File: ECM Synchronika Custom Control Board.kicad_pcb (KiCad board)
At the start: 2 copper layers, 17 parts, among them J1 Screw_Terminal_01x03, U1 AP2112K-3.3

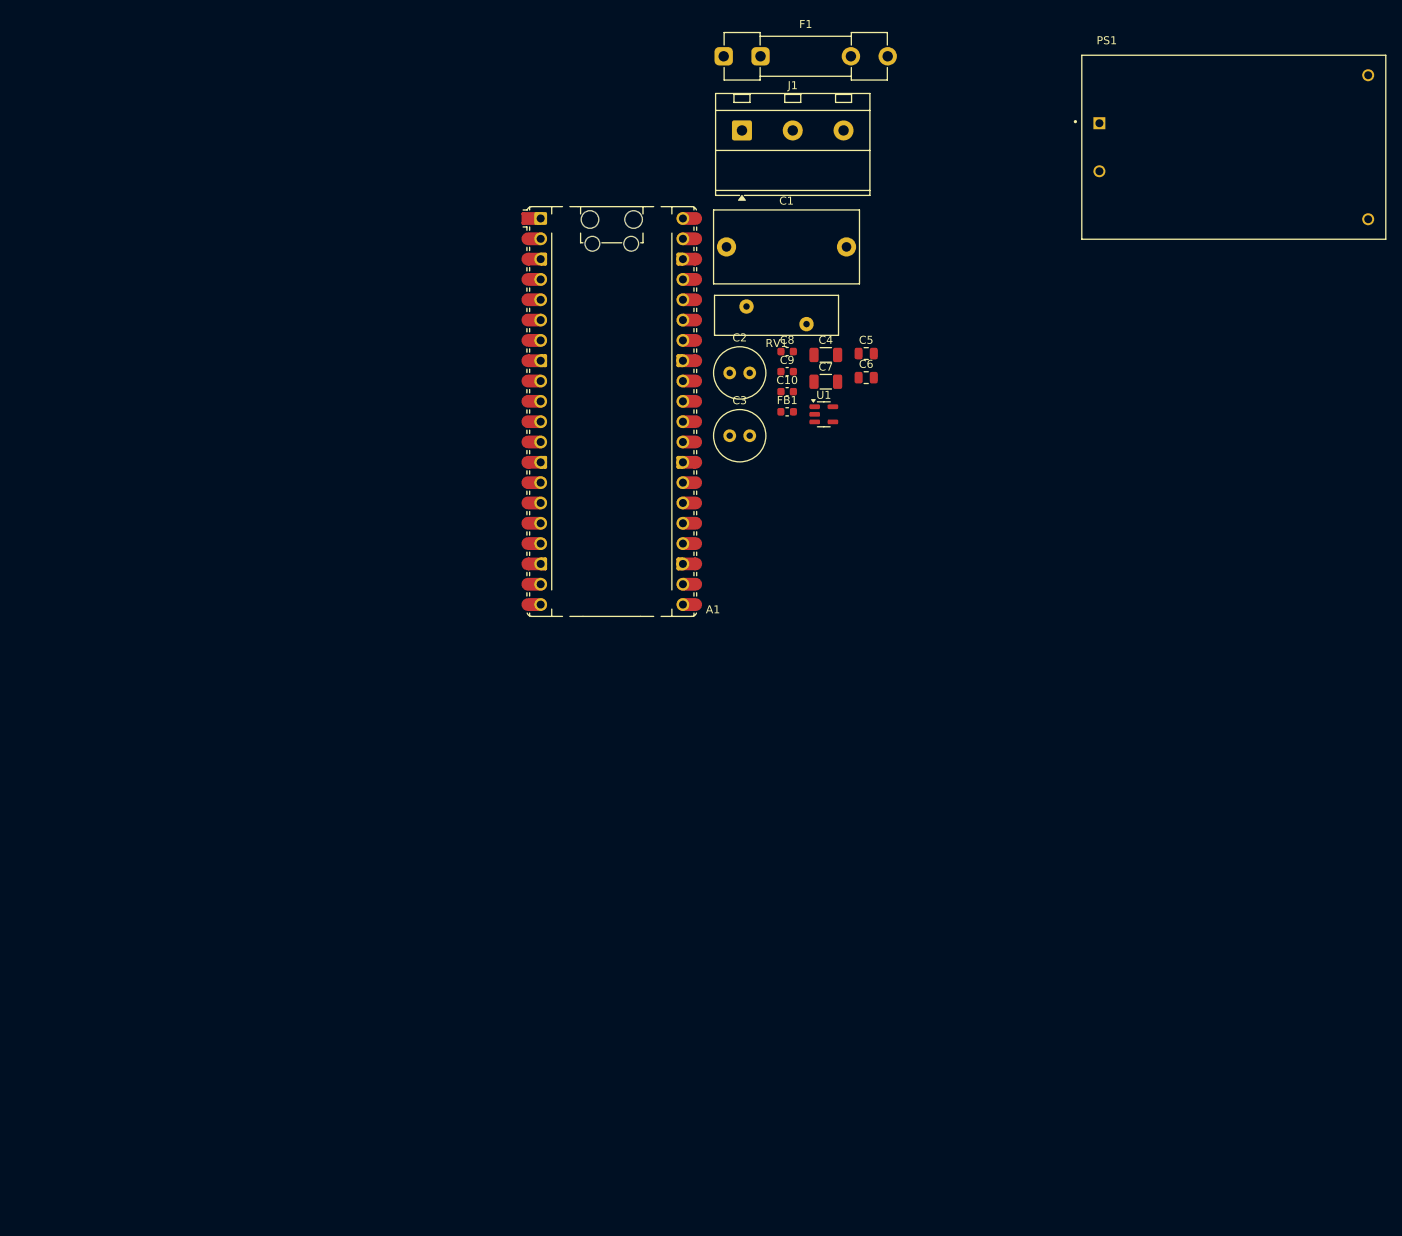
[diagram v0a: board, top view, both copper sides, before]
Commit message: Update KiCad project files
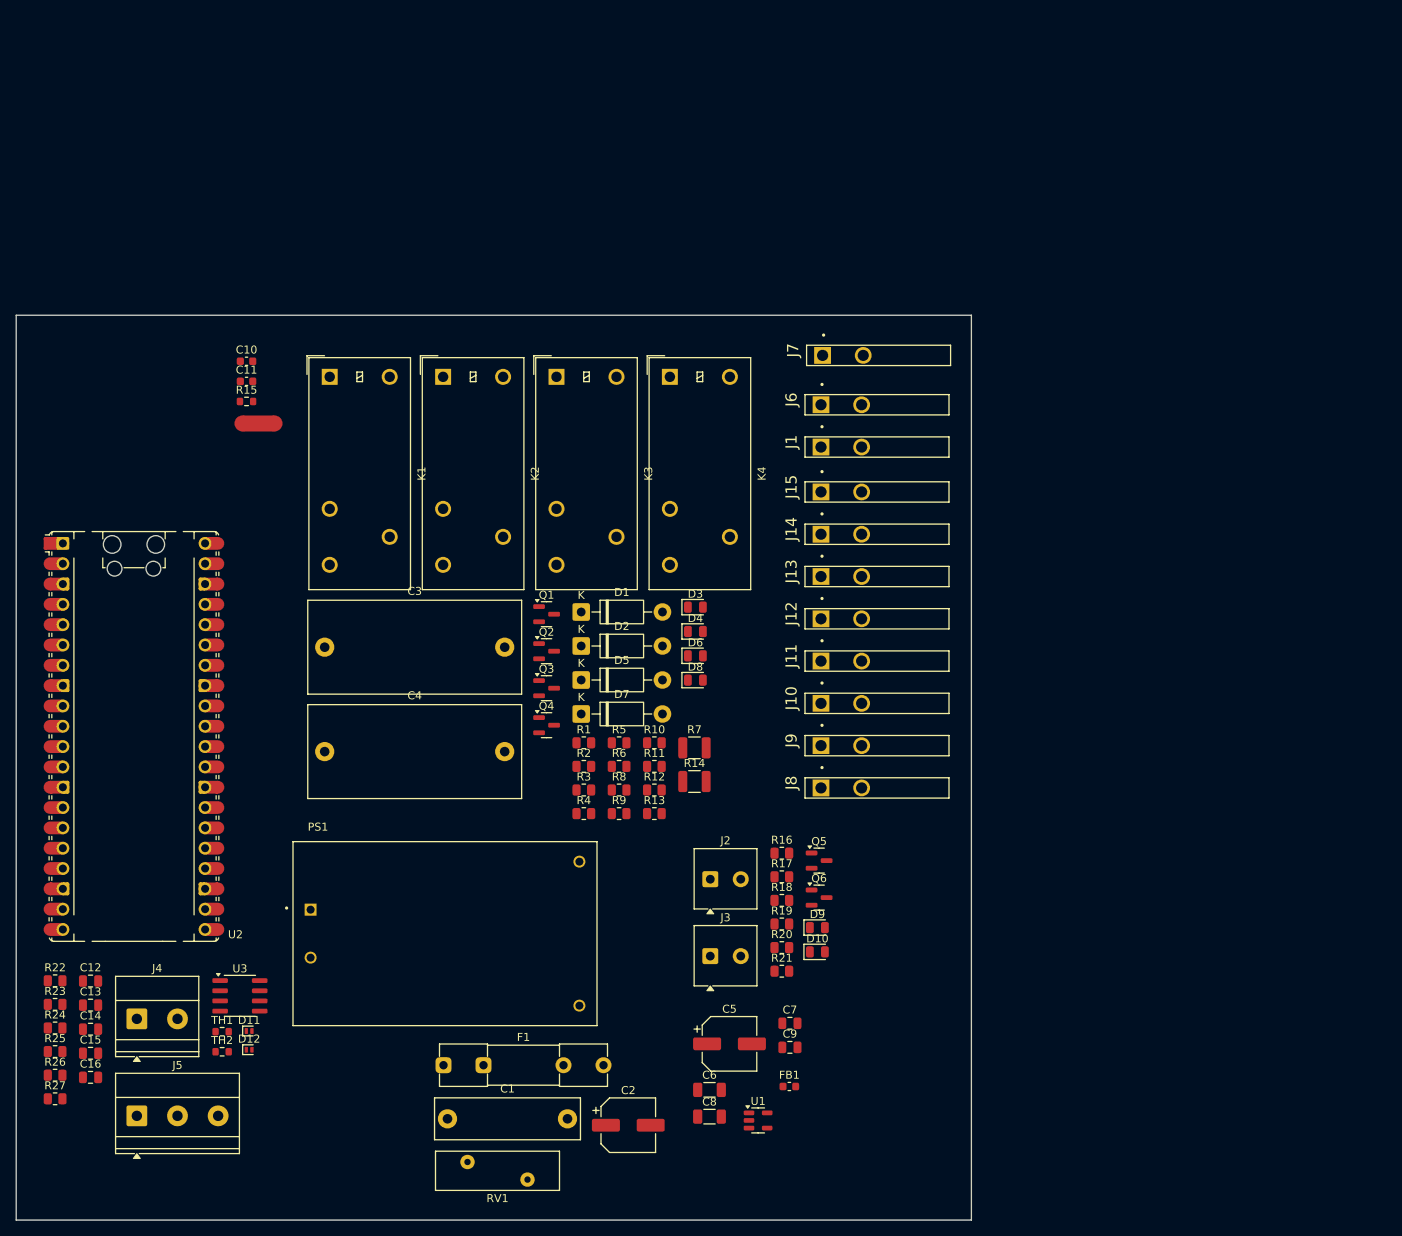
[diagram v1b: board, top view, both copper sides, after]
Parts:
- removed A1: RaspberryPi_Pico, Module:RaspberryPi_Pico_Common_Unspecified
- added C11: 100n, Capacitor_SMD:C_0603_1608Metric, F.Cu at (78.4, 87.6)
- added C12: 100n, Capacitor_SMD:C_0805_2012Metric, F.Cu at (58.9, 162.5)
- added C13: 100n, Capacitor_SMD:C_0805_2012Metric, F.Cu at (58.9, 165.5)
- added C14: 10n, Capacitor_SMD:C_0805_2012Metric, F.Cu at (58.9, 168.5)
- added C15: 100n, Capacitor_SMD:C_0805_2012Metric, F.Cu at (58.9, 171.6)
- added C16: 100n, Capacitor_SMD:C_0805_2012Metric, F.Cu at (58.9, 174.6)
- added D1: 1N4007, Diode_THT:D_DO-41_SOD81_P10.16mm_Horizontal, F.Cu at (120.2, 116.4)
- added D10: LED, LED_SMD:LED_0805_2012Metric, F.Cu at (149.8, 158.9)
- added D11: PESD5V0S1UL, Diode_SMD:D_SOD-882, F.Cu at (78.7, 168.8)
- added D12: PESD5V0S1UL, Diode_SMD:D_SOD-882, F.Cu at (78.7, 171.1)
- added D2: 1N4007, Diode_THT:D_DO-41_SOD81_P10.16mm_Horizontal, F.Cu at (120.2, 120.6)
- added D3: LED, LED_SMD:LED_0805_2012Metric, F.Cu at (134.5, 115.8)
- added D4: LED, LED_SMD:LED_0805_2012Metric, F.Cu at (134.5, 118.8)
- added D5: 1N4007, Diode_THT:D_DO-41_SOD81_P10.16mm_Horizontal, F.Cu at (120.2, 124.9)
- added D6: LED, LED_SMD:LED_0805_2012Metric, F.Cu at (134.5, 121.9)
- added D7: 1N4007, Diode_THT:D_DO-41_SOD81_P10.16mm_Horizontal, F.Cu at (120.2, 129.1)
- added D8: LED, LED_SMD:LED_0805_2012Metric, F.Cu at (134.5, 124.9)
- added D9: LED, LED_SMD:LED_0805_2012Metric, F.Cu at (149.8, 155.8)
- added J10: 928814-1, 6.3mm spade:TE_928814-1, F.Cu at (150.2, 127.8)
- added J11: 928814-1, 6.3mm spade:TE_928814-1, F.Cu at (150.2, 122.5)
- added J12: 928814-1, 6.3mm spade:TE_928814-1, F.Cu at (150.2, 117.2)
- added J13: 928814-1, 6.3mm spade:TE_928814-1, F.Cu at (150.2, 112.0)
- added J14: 928814-1, 6.3mm spade:TE_928814-1, F.Cu at (150.2, 106.7)
- added J15: 928814-1, 6.3mm spade:TE_928814-1, F.Cu at (150.2, 101.4)
- added J2: Screw_Terminal_01x02, TerminalBlock_Phoenix:TerminalBlock_Phoenix_MKDS-1-2-3.81_1x02_P3.81mm_Horizontal, F.Cu at (136.4, 149.8)
- added J3: Screw_Terminal_01x02, TerminalBlock_Phoenix:TerminalBlock_Phoenix_MKDS-1-2-3.81_1x02_P3.81mm_Horizontal, F.Cu at (136.4, 159.4)
- added J4: Screw_Terminal_01x02, TerminalBlock_Phoenix:TerminalBlock_Phoenix_MKDS-1,5-2-5.08_1x02_P5.08mm_Horizontal, F.Cu at (64.7, 167.3)
- added J5: Screw_Terminal_01x03, TerminalBlock_Phoenix:TerminalBlock_Phoenix_MKDS-1,5-3-5.08_1x03_P5.08mm_Horizontal, F.Cu at (64.7, 179.4)
- added J6: 928814-1, 6.3mm spade:TE_928814-1, F.Cu at (150.2, 90.5)
- added J7: 928814-1, 6.3mm spade:TE_928814-1, F.Cu at (150.4, 84.3)
- added J8: 928814-1, 6.3mm spade:TE_928814-1, F.Cu at (150.2, 138.4)
- added J9: 928814-1, 6.3mm spade:TE_928814-1, F.Cu at (150.2, 133.1)
- added K1: G2RL-1-H, Relay_THT:Relay_SPDT_Omron_G2RL-1, F.Cu at (88.8, 87.0)
- added K2: G2RL-1-H, Relay_THT:Relay_SPDT_Omron_G2RL-1, F.Cu at (103.0, 87.0)
- added K3: G2RL-1-H, Relay_THT:Relay_SPDT_Omron_G2RL-1, F.Cu at (117.1, 87.0)
- added K4: G2RL-1-H, Relay_THT:Relay_SPDT_Omron_G2RL-1, F.Cu at (131.3, 87.0)
- added NT1: NetTie_2, NetTie:NetTie-2_SMD_Pad2.0mm, F.Cu at (79.9, 92.8)
- added Q1: MMBT2222A, Package_TO_SOT_SMD:SOT-23, F.Cu at (115.9, 116.7)
- added Q2: MMBT2222A, Package_TO_SOT_SMD:SOT-23, F.Cu at (115.9, 121.3)
- added Q3: MMBT2222A, Package_TO_SOT_SMD:SOT-23, F.Cu at (115.9, 125.9)
- added Q4: MMBT2222A, Package_TO_SOT_SMD:SOT-23, F.Cu at (115.9, 130.5)
- added Q5: MMBT2222A, Package_TO_SOT_SMD:SOT-23, F.Cu at (150.0, 147.5)
- added Q6: MMBT2222A, Package_TO_SOT_SMD:SOT-23, F.Cu at (150.0, 152.1)
- added R1: 1K, Resistor_SMD:R_0805_2012Metric, F.Cu at (120.6, 132.7)
- added R10: 1K, Resistor_SMD:R_0805_2012Metric, F.Cu at (129.4, 132.7)
- added R11: 470, Resistor_SMD:R_0805_2012Metric, F.Cu at (129.4, 135.7)
- added R12: 10K, Resistor_SMD:R_0805_2012Metric, F.Cu at (129.4, 138.6)
- added R13: 10K, Resistor_SMD:R_0805_2012Metric, F.Cu at (129.4, 141.6)
- added R14: 100, Resistor_SMD:R_1210_3225Metric, F.Cu at (134.4, 137.6)
- added R15: 10K, Resistor_SMD:R_0603_1608Metric, F.Cu at (78.4, 90.1)
- added R16: 1K, Resistor_SMD:R_0805_2012Metric, F.Cu at (145.3, 146.5)
- added R17: 10K, Resistor_SMD:R_0805_2012Metric, F.Cu at (145.3, 149.5)
- added R18: 1K, Resistor_SMD:R_0805_2012Metric, F.Cu at (145.3, 152.4)
- added R19: 1K, Resistor_SMD:R_0805_2012Metric, F.Cu at (145.3, 155.4)
- added R2: 1K, Resistor_SMD:R_0805_2012Metric, F.Cu at (120.6, 135.7)
- added R20: 10K, Resistor_SMD:R_0805_2012Metric, F.Cu at (145.3, 158.3)
- added R21: 1K, Resistor_SMD:R_0805_2012Metric, F.Cu at (145.3, 161.3)
- added R22: 1K, Resistor_SMD:R_0805_2012Metric, F.Cu at (54.5, 162.5)
- added R23: 3.3K, Resistor_SMD:R_0805_2012Metric, F.Cu at (54.5, 165.4)
- added R24: 1.2K, Resistor_SMD:R_0805_2012Metric, F.Cu at (54.5, 168.4)
- added R25: 1K, Resistor_SMD:R_0805_2012Metric, F.Cu at (54.5, 171.3)
- added R26: 4.7K, Resistor_SMD:R_0805_2012Metric, F.Cu at (54.5, 174.3)
- added R27: 10K, Resistor_SMD:R_0805_2012Metric, F.Cu at (54.5, 177.2)
- added R3: 470, Resistor_SMD:R_0805_2012Metric, F.Cu at (120.6, 138.6)
- added R4: 470, Resistor_SMD:R_0805_2012Metric, F.Cu at (120.6, 141.6)
- added R5: 10K, Resistor_SMD:R_0805_2012Metric, F.Cu at (125.0, 132.7)
- added R6: 10K, Resistor_SMD:R_0805_2012Metric, F.Cu at (125.0, 135.7)
- added R7: 100, Resistor_SMD:R_1210_3225Metric, F.Cu at (134.4, 133.4)
- added R8: 1K, Resistor_SMD:R_0805_2012Metric, F.Cu at (125.0, 138.6)
- added R9: 470, Resistor_SMD:R_0805_2012Metric, F.Cu at (125.0, 141.6)
- added TH1: 50k NTC, Resistor_SMD:R_0603_1608Metric, F.Cu at (75.3, 168.9)
- added TH2: 50k NTC, Resistor_SMD:R_0603_1608Metric, F.Cu at (75.3, 171.4)
- added U2: RaspberryPi_Pico, Module:RaspberryPi_Pico_Common_Unspecified, F.Cu at (64.3, 131.9)
- added U3: MAX31855KASA, Package_SO:SOIC-8_3.9x4.9mm_P1.27mm, F.Cu at (77.6, 164.4)
- C1: footprint Capacitor_THT:C_Rect_L18.0mm_W9.0mm_P15.00mm_FKS3_FKP3 -> Capacitor_THT:C_Rect_L18.0mm_W5.0mm_P15.00mm_FKS3_FKP3
- C10: value 10u -> 100n
- C2: value C -> 100u; footprint Capacitor_THT:C_Radial_D6.3mm_H7.0mm_P2.50mm -> Capacitor_SMD:CP_Elec_6.3x5.9
- C3: value 100u -> 100n; footprint Capacitor_THT:C_Radial_D6.3mm_H7.0mm_P2.50mm -> Capacitor_THT:C_Rect_L26.5mm_W11.5mm_P22.50mm_MKS4
- C4: value 47u -> 100n; footprint Capacitor_SMD:C_1206_3216Metric -> Capacitor_THT:C_Rect_L26.5mm_W11.5mm_P22.50mm_MKS4
- C5: value 100n -> 100u; footprint Capacitor_SMD:C_0805_2012Metric -> Capacitor_SMD:CP_Elec_6.3x5.9
- C6: value 100n -> 47u; footprint Capacitor_SMD:C_0805_2012Metric -> Capacitor_SMD:C_1206_3216Metric
- C7: value 22U -> 100n; footprint Capacitor_SMD:C_1206_3216Metric -> Capacitor_SMD:C_0805_2012Metric
- C8: value 100n -> 22U; footprint Capacitor_SMD:C_0603_1608Metric -> Capacitor_SMD:C_1206_3216Metric
- C9: footprint Capacitor_SMD:C_0603_1608Metric -> Capacitor_SMD:C_0805_2012Metric
- F1: value Fuse -> Fuse_Small; footprint Fuse:Fuseholder_Clip-5x20mm_Littelfuse_100_Inline_P20.50x4.60mm_D1.30mm_Horizontal -> Fuse:Fuseholder_Clip-5x20mm_Littelfuse_111_Inline_P20.00x5.00mm_D1.05mm_Horizontal
- J1: value Screw_Terminal_01x03 -> 928814-1; footprint TerminalBlock_MetzConnect:TerminalBlock_MetzConnect_Type701_RT11L03HGLU_1x03_P6.35mm_Horizontal -> 6.3mm spade:TE_928814-1
- PS1: footprint HLK-5M05:CONV_HLK-5M05 -> HLK_5M05:CONV_HLK-5M05
- RV1: footprint Varistor:RV_Disc_D15.5mm_W5mm_P7.5mm -> Varistor:RV_Disc_D15.5mm_W4.9mm_P7.5mm
- moved PS1 139.2 mm to (103.2, 156.6)
- moved F1 130.9 mm to (103.0, 173.0)
- moved C1 114.4 mm to (103.5, 179.7)
- moved RV1 112.5 mm to (106.0, 185.1)
- moved C8 96.1 mm to (136.3, 179.5)
- moved C2 94.9 mm to (126.1, 180.5)
- moved C6 91.2 mm to (136.3, 176.1)
- moved U1 88.6 mm to (142.3, 179.9)
- moved C5 88.0 mm to (138.8, 170.4)
- moved C9 84.5 mm to (146.3, 170.8)
- moved FB1 84.3 mm to (146.2, 175.7)
- moved C7 80.3 mm to (146.3, 167.8)
- moved C4 79.9 mm to (88.2, 133.8)
- moved C10 67.7 mm to (78.4, 85.1)
- moved C3 57.1 mm to (88.2, 120.8)
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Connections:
- C1 pad 1: unconnected-(C1-Pad1) -> /HV_INPUT + PROTECTION/L_FUSED
- C1 pad 2: unconnected-(C1-Pad2) -> /HV_INPUT + PROTECTION/NEUTRAL
- C10 pad 1: unconnected-(C10-Pad1) -> GND
- C10 pad 2: unconnected-(C10-Pad2) -> +5v
- C2 pad 1: unconnected-(C2-Pad1) -> +5v
- C2 pad 2: unconnected-(C2-Pad2) -> GND
- C3 pad 1: unconnected-(C3-Pad1) -> /Relays+RC SNUBBER/PUMP_LOAD
- C3 pad 2: unconnected-(C3-Pad2) -> Net-(C3-Pad2)
- C4 pad 1: unconnected-(C4-Pad1) -> Net-(C4-Pad1)
- C4 pad 2: unconnected-(C4-Pad2) -> /HV_INPUT + PROTECTION/L_FUSED
- C5 pad 1: unconnected-(C5-Pad1) -> +5v
- C5 pad 2: unconnected-(C5-Pad2) -> GND
- C6 pad 1: unconnected-(C6-Pad1) -> Net-(U1-VOUT)
- C6 pad 2: unconnected-(C6-Pad2) -> GND
- C7 pad 1: unconnected-(C7-Pad1) -> Net-(U1-VOUT)
- C7 pad 2: unconnected-(C7-Pad2) -> GND
- C8 pad 1: unconnected-(C8-Pad1) -> Net-(C8-Pad1)
- C8 pad 2: unconnected-(C8-Pad2) -> GND
- C9 pad 1: unconnected-(C9-Pad1) -> ADC-REF
- C9 pad 2: unconnected-(C9-Pad2) -> GND
- F1 pad 1: unconnected-(F1-Pad1) -> /HV_INPUT + PROTECTION/LIVE
- F1 pad 2: unconnected-(F1-Pad2) -> /HV_INPUT + PROTECTION/L_FUSED
- FB1 pad 1: unconnected-(FB1-Pad1) -> Net-(C8-Pad1)
- FB1 pad 2: unconnected-(FB1-Pad2) -> ADC-REF
- J1 pad 1: unconnected-(J1-Pin_1-Pad1) -> /HV_INPUT + PROTECTION/NEUTRAL
- J1 pad 2: unconnected-(J1-Pin_2-Pad2) -> (no net)
- PS1 pad 1: unconnected-(PS1-AC1-Pad1) -> /HV_INPUT + PROTECTION/L_FUSED
- PS1 pad 2: unconnected-(PS1-AC2-Pad2) -> /HV_INPUT + PROTECTION/NEUTRAL
- PS1 pad 3: unconnected-(PS1--VO-Pad3) -> GND
- PS1 pad 4: unconnected-(PS1-+VO-Pad4) -> +5v
- RV1 pad 1: unconnected-(RV1-Pad1) -> /HV_INPUT + PROTECTION/LIVE
- RV1 pad 2: unconnected-(RV1-Pad2) -> /HV_INPUT + PROTECTION/NEUTRAL
- U1 pad 1: unconnected-(U1-VIN-Pad1) -> +5v
- U1 pad 2: unconnected-(U1-GND-Pad2) -> GND
- U1 pad 3: unconnected-(U1-EN-Pad3) -> 3V3-EN
- U1 pad 5: unconnected-(U1-VOUT-Pad5) -> Net-(U1-VOUT)
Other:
- board outline added: 119.4 x 113.1 mm
